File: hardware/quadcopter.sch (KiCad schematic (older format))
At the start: 33 parts, among them J1 CONN-MOTOR, J2 CONN-MOTOR, J3 CONN-MOTOR, J4 CONN-MOTOR, J5 Conn_ARM_JTAG_SWD_20, J6 GIMBAL, K1 BATTERY, U1 ESC, U2 ESP-WROOM-32-board, U3 LM2936-5.0, U4 10DOF, U5 SI4432-board, U6 HC-SR04, U7 GPS

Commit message: [hardware] Generate netlist
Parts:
- C1, C3: footprint (none) -> Capacitor_THT:CP_Radial_D10.0mm_P5.00mm
- C2: footprint (none) -> Capacitor_SMD:C_1206_3216Metric_Pad1.42x1.75mm_HandSolder
- D1, D2: footprint (none) -> LED_SMD:LED_1206_3216Metric_Pad1.42x1.75mm_HandSolder
- J1, J2, J3, J4: footprint (none) -> Connector_PinHeader_2.54mm:PinHeader_1x03_P2.54mm_Vertical
- J5: footprint (none) -> Connector_IDC:IDC-Header_2x10_P2.54mm_Horizontal
- J6: footprint (none) -> quadcopter:GIMBAL
- JP1, K1: footprint (none) -> Connector_PinHeader_2.54mm:PinHeader_1x02_P2.54mm_Vertical
- R1, R10, R11, R12, R13, R2, R3, R4, R5, R6, R7, R8, R9: footprint (none) -> Resistor_SMD:R_1206_3216Metric_Pad1.42x1.75mm_HandSolder
- U1: footprint (none) -> quadcopter:ESC
- U2: footprint (none) -> quadcopter:ESP32-VROOM-board
- U3: footprint (none) -> Package_TO_SOT_SMD:TO-263-2
- U4: footprint (none) -> quadcopter:10DOF
- U5: footprint (none) -> quadcopter:SI4432-board
- U6: footprint (none) -> quadcopter:HC-SR04
- U7: footprint (none) -> quadcopter:GPS
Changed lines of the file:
@@
 F 0 "U2" H 3450 2600 60  0000 C CNN
 F 1 "ESP-WROOM-32-board" H 3950 300 60  0000 C CNN
-F 2 "" H 3200 1900 60  0001 C CNN
+F 2 "quadcopter:ESP32-VROOM-board" H 3200 1900 60  0001 C CNN
 F 3 "" H 3200 1900 60  0001 C CNN
 	1    3200 1900
@@
 F 0 "K1" H 7550 5950 60  0000 C CNN
 F 1 "BATTERY" H 7700 5450 60  0000 C CNN
-F 2 "" H 7600 5700 60  0001 C CNN
+F 2 "Connector_PinHeader_2.54mm:PinHeader_1x02_P2.54mm_Vertical" H 7600 5700 60  0001 C CNN
 F 3 "" H 7600 5700 60  0001 C CNN
 	1    7650 5700
@@
 F 0 "U4" H 6450 2150 60  0000 C CNN
 F 1 "10DOF" H 6800 1150 60  0000 C CNN
-F 2 "" H 6500 1500 60  0001 C CNN
+F 2 "quadcopter:10DOF" H 6500 1500 60  0001 C CNN
 F 3 "" H 6500 1500 60  0001 C CNN
 	1    6600 1650
@@
 F 0 "J1" H 1350 5100 60  0000 C CNN
 F 1 "CONN-MOTOR" H 1650 4500 60  0000 C CNN
-F 2 "" H 1350 4700 60  0001 C CNN
+F 2 "Connector_PinHeader_2.54mm:PinHeader_1x03_P2.54mm_Vertical" H 1350 4700 60  0001 C CNN
 F 3 "" H 1350 4700 60  0001 C CNN
 	1    1400 4800
@@
 F 0 "J2" H 1350 5900 60  0000 C CNN
 F 1 "CONN-MOTOR" H 1650 5300 60  0000 C CNN
-F 2 "" H 1350 5500 60  0001 C CNN
+F 2 "Connector_PinHeader_2.54mm:PinHeader_1x03_P2.54mm_Vertical" H 1350 5500 60  0001 C CNN
 F 3 "" H 1350 5500 60  0001 C CNN
 	1    1400 5600
@@
 F 0 "J3" H 1350 6650 60  0000 C CNN
 F 1 "CONN-MOTOR" H 1650 6050 60  0000 C CNN
-F 2 "" H 1350 6250 60  0001 C CNN
+F 2 "Connector_PinHeader_2.54mm:PinHeader_1x03_P2.54mm_Vertical" H 1350 6250 60  0001 C CNN
 F 3 "" H 1350 6250 60  0001 C CNN
 	1    1400 6350
@@
 F 0 "J4" H 1350 7450 60  0000 C CNN
 F 1 "CONN-MOTOR" H 1650 6850 60  0000 C CNN
-F 2 "" H 1350 7050 60  0001 C CNN
+F 2 "Connector_PinHeader_2.54mm:PinHeader_1x03_P2.54mm_Vertical" H 1350 7050 60  0001 C CNN
 F 3 "" H 1350 7050 60  0001 C CNN
 	1    1400 7150
@@
 F 0 "U1" H 2550 6650 60  0000 C CNN
 F 1 "ESC" H 3150 5100 60  0000 C CNN
-F 2 "" H 2850 6600 60  0001 C CNN
+F 2 "quadcopter:ESC" H 2850 6600 60  0001 C CNN
 F 3 "" H 2850 6600 60  0001 C CNN
 	1    2900 5950
@@
 F 0 "J6" H 10000 3850 60  0000 C CNN
 F 1 "GIMBAL" H 10300 3150 60  0000 C CNN
-F 2 "" H 10050 3300 60  0001 C CNN
+F 2 "quadcopter:GIMBAL" H 10050 3300 60  0001 C CNN
 F 3 "" H 10050 3300 60  0001 C CNN
 	1    10100 3500
@@
 F 0 "U6" H 10000 1850 60  0000 C CNN
 F 1 "HC-SR04" H 10250 1100 60  0000 C CNN
-F 2 "" H 10200 1250 60  0001 C CNN
+F 2 "quadcopter:HC-SR04" H 10200 1250 60  0001 C CNN
 F 3 "" H 10200 1250 60  0001 C CNN
 	1    10150 1500
@@
 F 0 "U5" H 6500 4450 60  0000 C CNN
 F 1 "SI4432-board" H 7350 2900 60  0000 C CNN
-F 2 "" H 7050 3700 60  0001 C CNN
+F 2 "quadcopter:SI4432-board" H 7050 3700 60  0001 C CNN
 F 3 "" H 7050 3700 60  0001 C CNN
 	1    6950 3700
@@
 F 0 "U7" H 10200 5650 60  0000 C CNN
 F 1 "GPS" H 10450 4950 60  0000 C CNN
-F 2 "" H 10350 5150 60  0001 C CNN
+F 2 "quadcopter:GPS" H 10350 5150 60  0001 C CNN
 F 3 "" H 10350 5150 60  0001 C CNN
 	1    10350 5300
@@
 F 0 "C3" H 7075 5800 50  0000 L CNN
 F 1 "470u" H 7075 5600 50  0000 L CNN
-F 2 "" H 7088 5550 50  0001 C CNN
+F 2 "Capacitor_THT:CP_Radial_D10.0mm_P5.00mm" H 7088 5550 50  0001 C CNN
 F 3 "" H 7050 5700 50  0001 C CNN
 	1    7050 5700
@@
 F 0 "R11" V 9630 1600 50  0000 C CNN
 F 1 "10k" V 9550 1600 50  0000 C CNN
-F 2 "" V 9480 1600 50  0001 C CNN
+F 2 "Resistor_SMD:R_1206_3216Metric_Pad1.42x1.75mm_HandSolder" V 9480 1600 50  0001 C CNN
 F 3 "" H 9550 1600 50  0001 C CNN
 	1    9550 1600
@@
 F 0 "R8" V 9430 1800 50  0000 C CNN
 F 1 "20k" V 9350 1800 50  0000 C CNN
-F 2 "" V 9280 1800 50  0001 C CNN
+F 2 "Resistor_SMD:R_1206_3216Metric_Pad1.42x1.75mm_HandSolder" V 9280 1800 50  0001 C CNN
 F 3 "" H 9350 1800 50  0001 C CNN
 	1    9350 1800
@@
 F 0 "R12" V 9580 3600 50  0000 C CNN
 F 1 "10k" V 9500 3600 50  0000 C CNN
-F 2 "" V 9430 3600 50  0001 C CNN
+F 2 "Resistor_SMD:R_1206_3216Metric_Pad1.42x1.75mm_HandSolder" V 9430 3600 50  0001 C CNN
 F 3 "" H 9500 3600 50  0001 C CNN
 	1    9500 3600
@@
 F 0 "R9" V 9330 3800 50  0000 C CNN
 F 1 "20k" V 9250 3800 50  0000 C CNN
-F 2 "" V 9180 3800 50  0001 C CNN
+F 2 "Resistor_SMD:R_1206_3216Metric_Pad1.42x1.75mm_HandSolder" V 9180 3800 50  0001 C CNN
 F 3 "" H 9250 3800 50  0001 C CNN
 	1    9250 3800
@@
 F 0 "U3" H 5550 5625 50  0000 C CNN
 F 1 "LM2936-5.0" H 5700 5625 50  0000 L CNN
-F 2 "" H 5700 5725 50  0001 C CIN
+F 2 "Package_TO_SOT_SMD:TO-263-2" H 5700 5725 50  0001 C CIN
 F 3 "" H 5700 5450 50  0001 C CNN
 	1    5700 5500
@@
 F 0 "C2" H 6125 5800 50  0000 L CNN
 F 1 "470n" H 6125 5600 50  0000 L CNN
-F 2 "" H 6138 5550 50  0001 C CNN
+F 2 "Capacitor_SMD:C_1206_3216Metric_Pad1.42x1.75mm_HandSolder" H 6138 5550 50  0001 C CNN
 F 3 "" H 6100 5700 50  0001 C CNN
 	1    6100 5700
@@
 F 0 "C1" H 5225 5800 50  0000 L CNN
 F 1 "22u" H 5225 5600 50  0000 L CNN
-F 2 "" H 5238 5550 50  0001 C CNN
+F 2 "Capacitor_THT:CP_Radial_D10.0mm_P5.00mm" H 5238 5550 50  0001 C CNN
 F 3 "" H 5200 5700 50  0001 C CNN
 	1    5200 5700
@@
 F 0 "R7" V 9230 5400 50  0000 C CNN
 F 1 "20k" V 9150 5400 50  0000 C CNN
-F 2 "" V 9080 5400 50  0001 C CNN
+F 2 "Resistor_SMD:R_1206_3216Metric_Pad1.42x1.75mm_HandSolder" V 9080 5400 50  0001 C CNN
 F 3 "" H 9150 5400 50  0001 C CNN
 	1    9150 5400
@@
 F 0 "R10" V 9480 5200 50  0000 C CNN
 F 1 "10k" V 9400 5200 50  0000 C CNN
-F 2 "" V 9330 5200 50  0001 C CNN
+F 2 "Resistor_SMD:R_1206_3216Metric_Pad1.42x1.75mm_HandSolder" V 9330 5200 50  0001 C CNN
 F 3 "" H 9400 5200 50  0001 C CNN
 	1    9400 5200
@@
 F 0 "R6" V 6880 5900 50  0000 C CNN
 F 1 "10k" V 6800 5900 50  0000 C CNN
-F 2 "" V 6730 5900 50  0001 C CNN
+F 2 "Resistor_SMD:R_1206_3216Metric_Pad1.42x1.75mm_HandSolder" V 6730 5900 50  0001 C CNN
 F 3 "" H 6800 5900 50  0001 C CNN
 	1    6800 5900
@@
 F 0 "R5" V 6880 5500 50  0000 C CNN
 F 1 "30k" V 6800 5500 50  0000 C CNN
-F 2 "" V 6730 5500 50  0001 C CNN
+F 2 "Resistor_SMD:R_1206_3216Metric_Pad1.42x1.75mm_HandSolder" V 6730 5500 50  0001 C CNN
 F 3 "" H 6800 5500 50  0001 C CNN
 	1    6800 5500
@@
 F 0 "J5" H 1250 3700 50  0000 R CNN
 F 1 "Conn_ARM_JTAG_SWD_20" H 1250 3600 50  0000 R BNN
-F 2 "" H 1900 1800 50  0001 L TNN
+F 2 "Connector_IDC:IDC-Header_2x10_P2.54mm_Horizontal" H 1900 1800 50  0001 L TNN
 F 3 "" V 1100 1600 50  0001 C CNN
 	1    1450 2850
@@
 F 0 "JP1" H 1450 1900 50  0000 C CNN
 F 1 "Jumper" H 1450 1670 50  0000 C CNN
-F 2 "" H 1450 1750 50  0001 C CNN
+F 2 "Connector_PinHeader_2.54mm:PinHeader_1x02_P2.54mm_Vertical" H 1450 1750 50  0001 C CNN
 F 3 "" H 1450 1750 50  0001 C CNN
 	1    1450 1750
@@
 F 0 "R13" V 9830 5700 50  0000 C CNN
 F 1 "1k" V 9750 5700 50  0000 C CNN
-F 2 "" V 9680 5700 50  0001 C CNN
+F 2 "Resistor_SMD:R_1206_3216Metric_Pad1.42x1.75mm_HandSolder" V 9680 5700 50  0001 C CNN
 F 3 "" H 9750 5700 50  0001 C CNN
 	1    9750 5700
@@
 F 0 "D2" H 10000 6000 50  0000 C CNN
 F 1 "LED" H 10000 5800 50  0000 C CNN
-F 2 "" H 10000 5900 50  0001 C CNN
+F 2 "LED_SMD:LED_1206_3216Metric_Pad1.42x1.75mm_HandSolder" H 10000 5900 50  0001 C CNN
 F 3 "" H 10000 5900 50  0001 C CNN
 	1    10000 5900
@@
 F 0 "R2" V 6080 3100 50  0000 C CNN
 F 1 "0" V 6000 3100 50  0000 C CNN
-F 2 "" V 5930 3100 50  0001 C CNN
+F 2 "Resistor_SMD:R_1206_3216Metric_Pad1.42x1.75mm_HandSolder" V 5930 3100 50  0001 C CNN
 F 3 "" H 6000 3100 50  0001 C CNN
 	1    6000 3100
@@
 F 0 "R3" V 6080 3250 50  0000 C CNN
 F 1 "0" V 6000 3250 50  0000 C CNN
-F 2 "" V 5930 3250 50  0001 C CNN
+F 2 "Resistor_SMD:R_1206_3216Metric_Pad1.42x1.75mm_HandSolder" V 5930 3250 50  0001 C CNN
 F 3 "" H 6000 3250 50  0001 C CNN
 	1    6000 3250
@@
 F 0 "R4" V 6080 3400 50  0000 C CNN
 F 1 "0" V 6000 3400 50  0000 C CNN
-F 2 "" V 5930 3400 50  0001 C CNN
+F 2 "Resistor_SMD:R_1206_3216Metric_Pad1.42x1.75mm_HandSolder" V 5930 3400 50  0001 C CNN
 F 3 "" H 6000 3400 50  0001 C CNN
 	1    6000 3400
@@
 F 0 "R1" V 4980 5550 50  0000 C CNN
 F 1 "1k" V 4900 5550 50  0000 C CNN
-F 2 "" V 4830 5550 50  0001 C CNN
+F 2 "Resistor_SMD:R_1206_3216Metric_Pad1.42x1.75mm_HandSolder" V 4830 5550 50  0001 C CNN
 F 3 "" H 4900 5550 50  0001 C CNN
 	1    4900 5550
@@
 F 0 "D1" H 4900 6000 50  0000 C CNN
 F 1 "LED" H 4900 5800 50  0000 C CNN
-F 2 "" H 4900 5900 50  0001 C CNN
+F 2 "LED_SMD:LED_1206_3216Metric_Pad1.42x1.75mm_HandSolder" H 4900 5900 50  0001 C CNN
 F 3 "" H 4900 5900 50  0001 C CNN
 	1    4900 5900

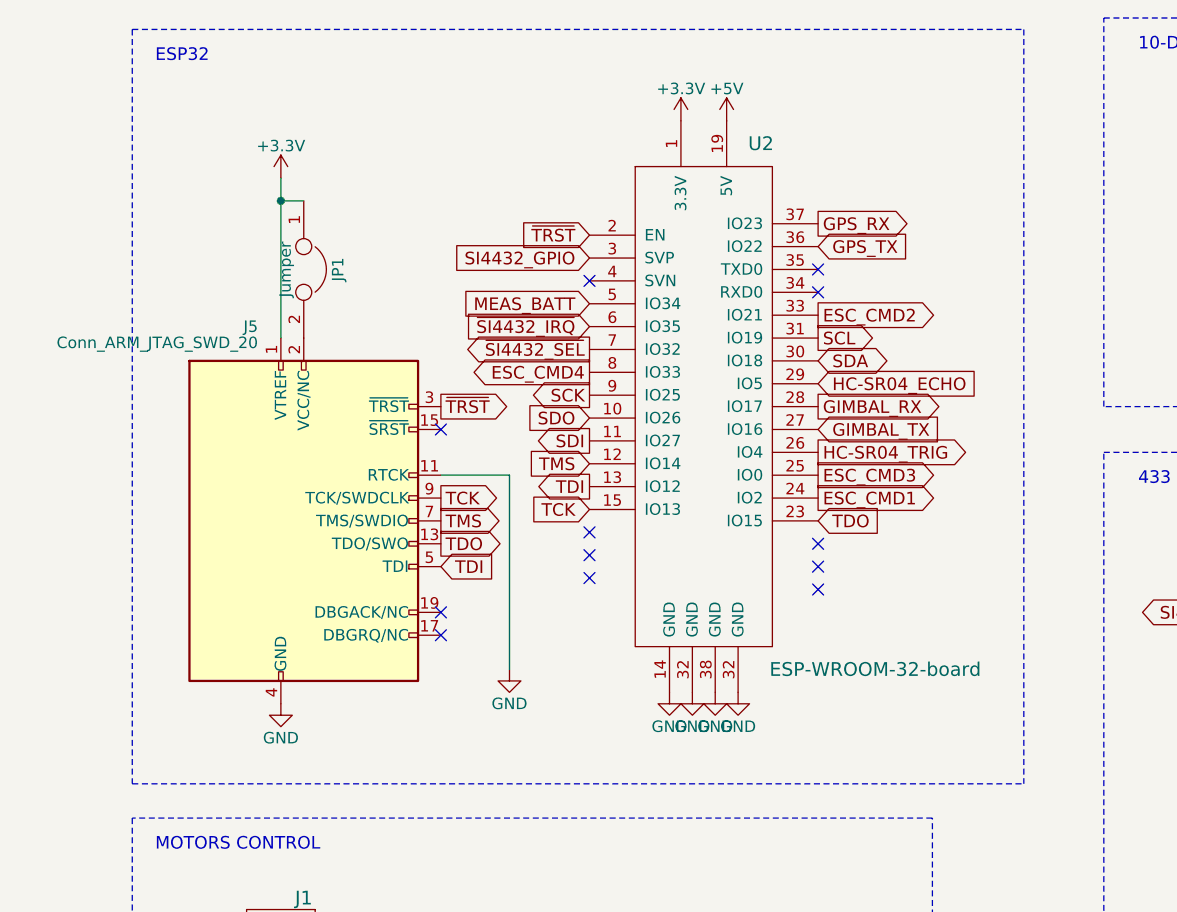
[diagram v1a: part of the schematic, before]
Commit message: [hardware] PCB 1.0
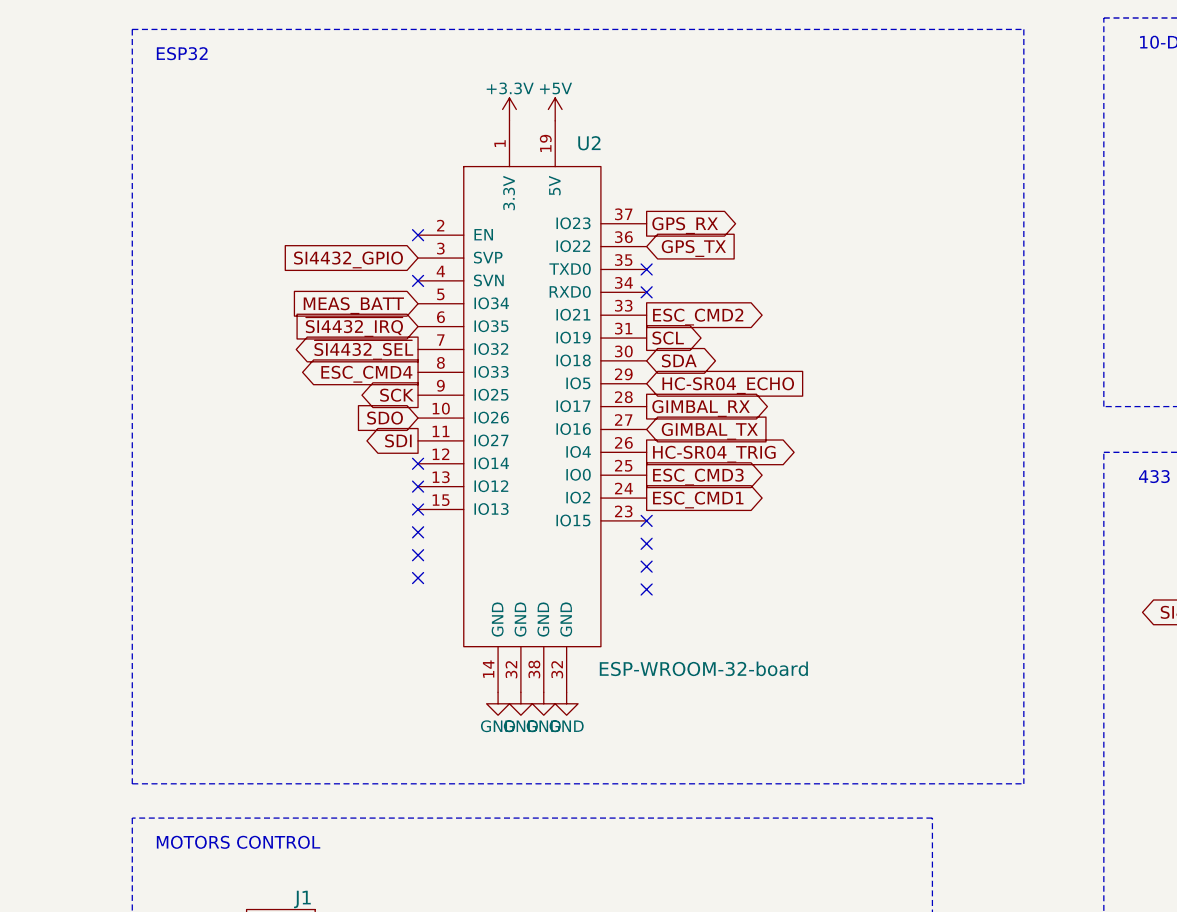
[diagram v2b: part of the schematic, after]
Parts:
- removed J5: Conn_ARM_JTAG_SWD_20, Connector_IDC:IDC-Header_2x10_P2.54mm_Horizontal, symbol quadcopter-rescue:Conn_ARM_JTAG_SWD_20
- removed JP1: Jumper, Connector_PinHeader_2.54mm:PinHeader_1x02_P2.54mm_Vertical, symbol quadcopter-rescue:Jumper
- C1: footprint Capacitor_THT:CP_Radial_D10.0mm_P5.00mm -> Capacitor_THT:CP_Radial_D5.0mm_P2.50mm
- J1, J2, J3, J4: footprint Connector_PinHeader_2.54mm:PinHeader_1x03_P2.54mm_Vertical -> quadcopter:motor-connector
- K1: footprint Connector_PinHeader_2.54mm:PinHeader_1x02_P2.54mm_Vertical -> quadcopter:battery-connector
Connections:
- net TCK: no longer names the net of U2.15 (IO13)
- net TDI: no longer names the net of U2.13 (IO12)
- net TDO: no longer names the net of U2.23 (IO15)
- net TMS: no longer names the net of U2.12 (IO14)
- net ~TRST: no longer names the net of U2.2 (EN)
- no-connect marks 16 -> 18
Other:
- moved on the sheet: U2
